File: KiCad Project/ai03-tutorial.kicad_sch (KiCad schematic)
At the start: 14 parts, among them SW1 SW_Push, U1 ATmega32U4-A, Y1 16MHz

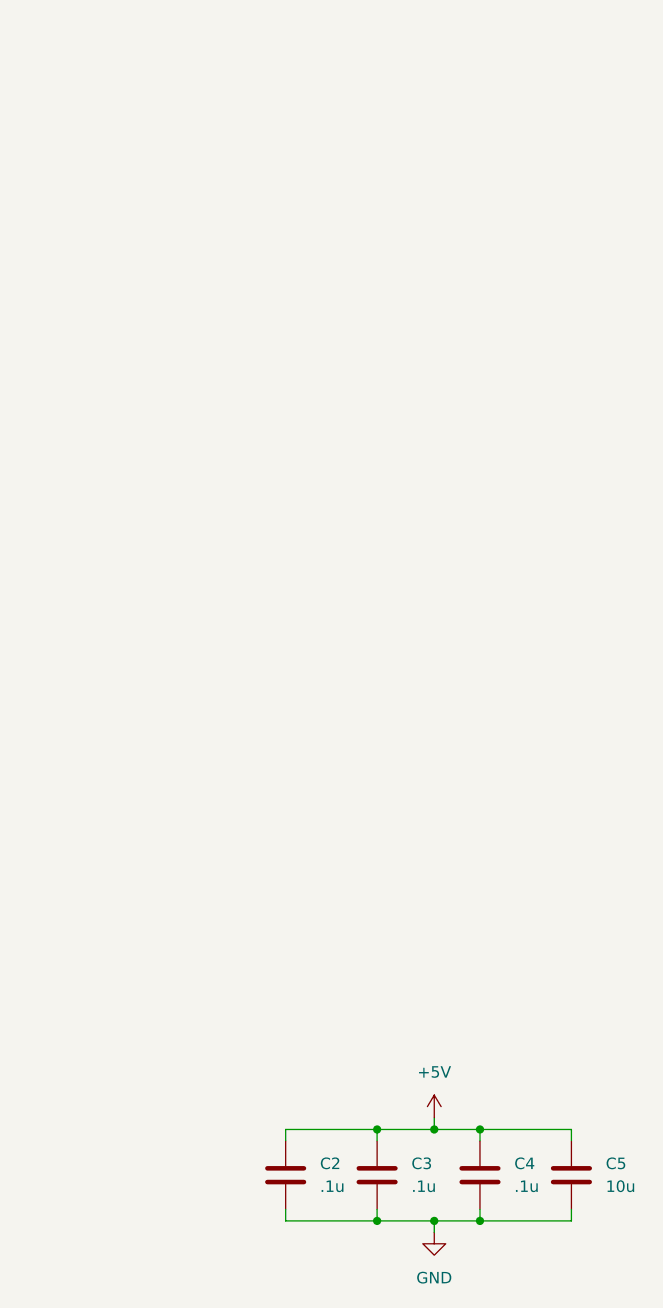
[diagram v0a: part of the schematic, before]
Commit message: Finished PCB guide part 4 - schematic.
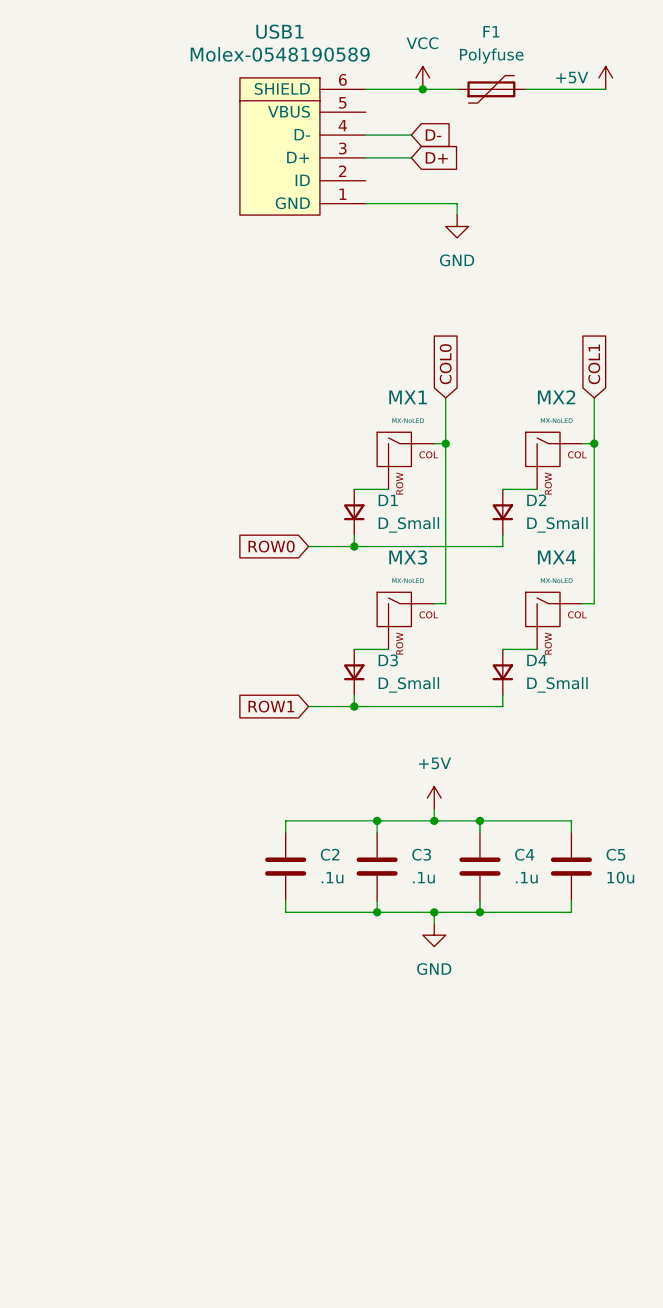
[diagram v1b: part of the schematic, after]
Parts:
- added D1, D2, D3, D4: D_Small, Diode_SMD:D_SOD-123, symbol Device:D_Small
- added F1: Polyfuse, Fuse:Fuse_1206_3216Metric, symbol Device:Polyfuse
- added MX1, MX2, MX3, MX4: MX-NoLED, MX_Alps_Hybrid:MX-1U-NoLED, symbol MX_Alps_Hybrid:MX-NoLED
- added USB1: Molex-0548190589, random-keyboard-parts:Molex-0548190589, symbol random-keyboard-parts:Molex-0548190589
- C1, C2, C3, C4, C5, C6, C7: footprint (none) -> Capacitor_SMD:C_0805_2012Metric
- R1, R2, R3, R4: footprint (none) -> Resistor_SMD:R_0805_2012Metric
- SW1: footprint (none) -> random-keyboard-parts:SKQG-1155865
- Y1: footprint (none) -> Crystal:Crystal_SMD_3225-4Pin_3.2x2.5mm
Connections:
- net +5V: now also F1.2
- net D+: now also USB1.3 (D+)
- net D-: now also USB1.4 (D-)
- net GND: now also USB1.1 (GND)
- new net: D1.2 (A), MX1.2 (ROW)
- new net: D3.2 (A), MX3.2 (ROW)
- new net: D4.2 (A), MX4.2 (ROW)
- new net: D2.2 (A), MX2.2 (ROW)
- new net COL0: MX1.1 (COL), MX3.1 (COL)
- new net COL1: MX2.1 (COL), MX4.1 (COL)
- new net ROW0: D1.1 (K), D2.1 (K)
- new net ROW1: D3.1 (K), D4.1 (K)
- new net VCC: F1.1, USB1.6 (SHIELD)
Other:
- moved on the sheet: C2, C3, C4, C5
